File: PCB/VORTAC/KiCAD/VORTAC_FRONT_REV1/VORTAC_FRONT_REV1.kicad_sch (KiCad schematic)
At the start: 5 parts, among them J1 Conn_02x02_Odd_Even, J2 Conn_02x03_Odd_Even, J3 Conn_01x07

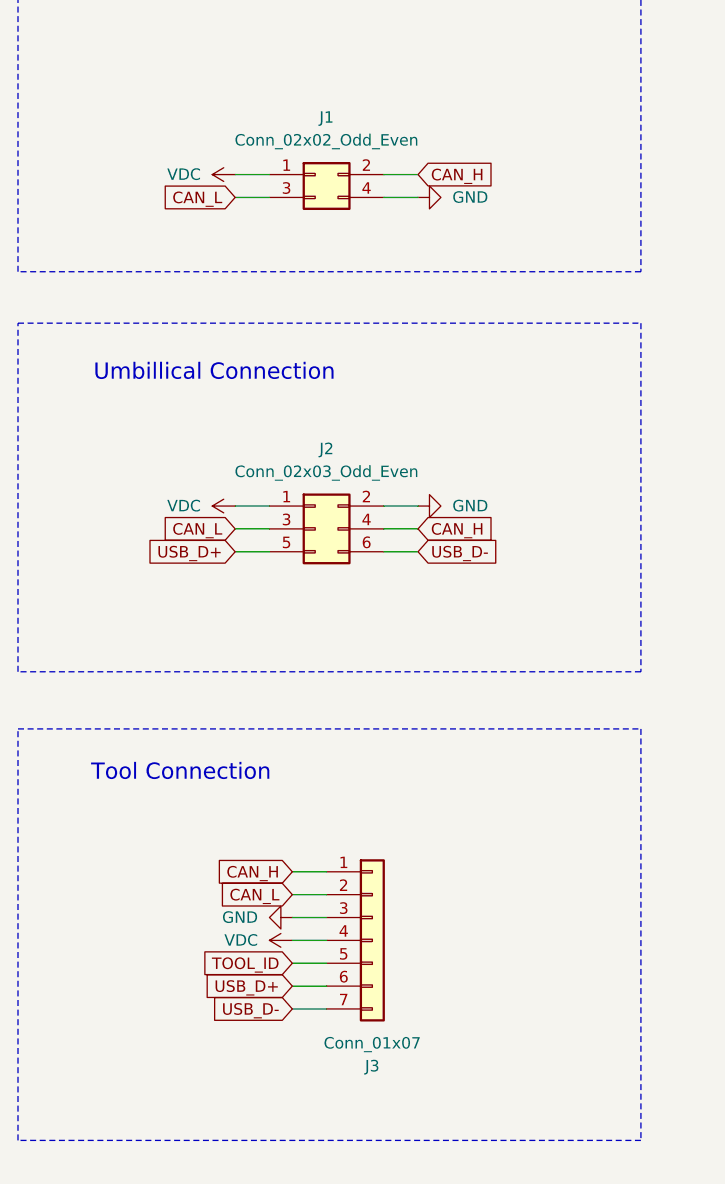
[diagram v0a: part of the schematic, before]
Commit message: No Body knows.... The trouble I've seen
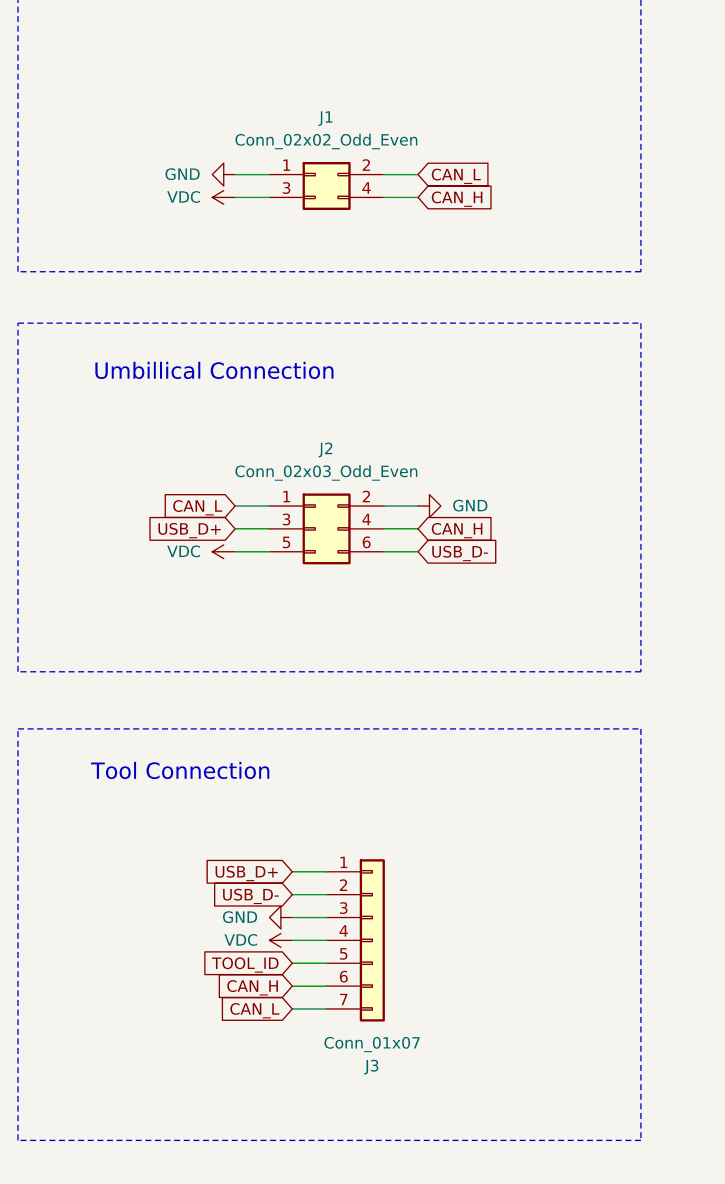
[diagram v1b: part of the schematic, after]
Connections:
- net CAN_H: now also J1.4 (Pin_4), J3.6 (Pin_6); no longer J1.2 (Pin_2), J3.1 (Pin_1)
- net CAN_L: now also J1.2 (Pin_2), J2.1 (Pin_1), J3.7 (Pin_7); no longer J1.3 (Pin_3), J2.3 (Pin_3), J3.2 (Pin_2)
- net GND: now also J1.1 (Pin_1); no longer J1.4 (Pin_4)
- net USB_D+: now also J2.3 (Pin_3), J3.1 (Pin_1); no longer J2.5 (Pin_5), J3.6 (Pin_6)
- net USB_D-: now also J3.2 (Pin_2); no longer J3.7 (Pin_7)
- net VDC: now also J1.3 (Pin_3), J2.5 (Pin_5); no longer J1.1 (Pin_1), J2.1 (Pin_1)

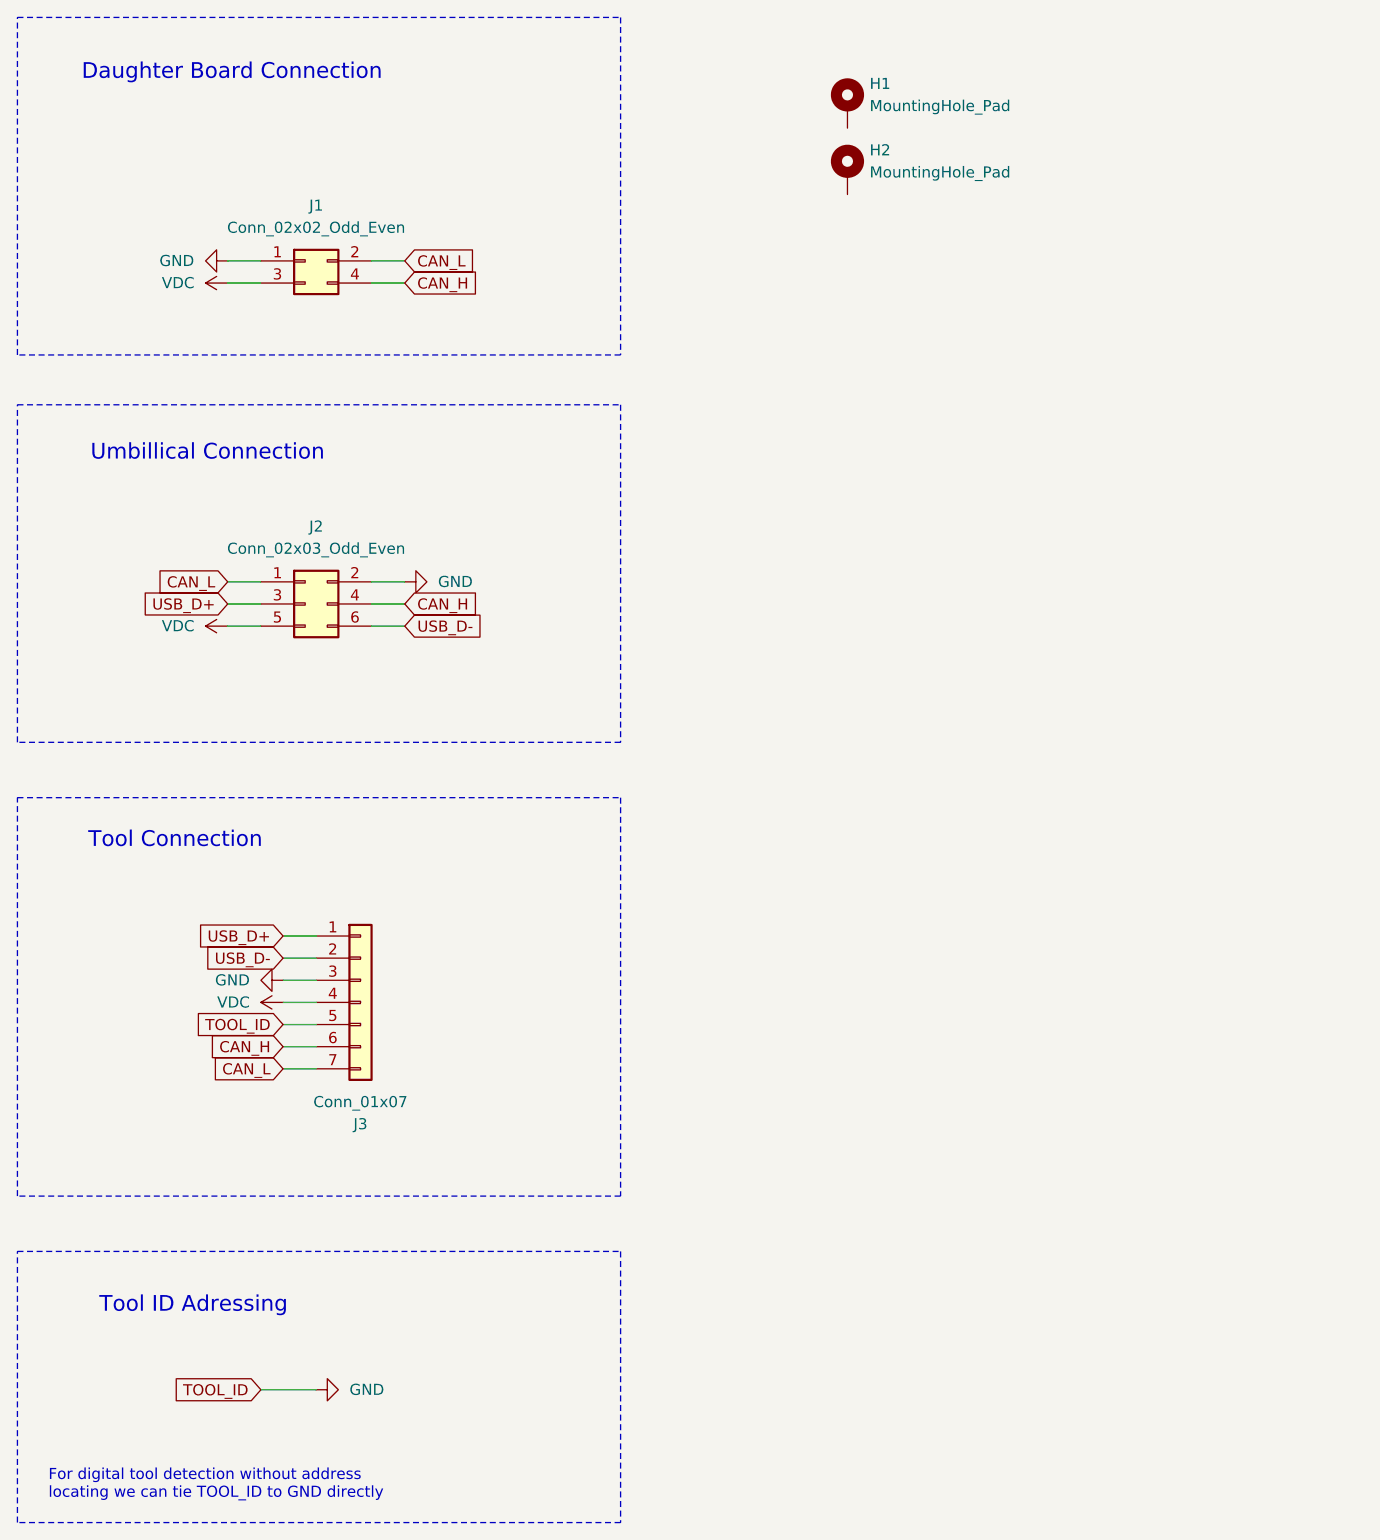
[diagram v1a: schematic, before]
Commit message: FML
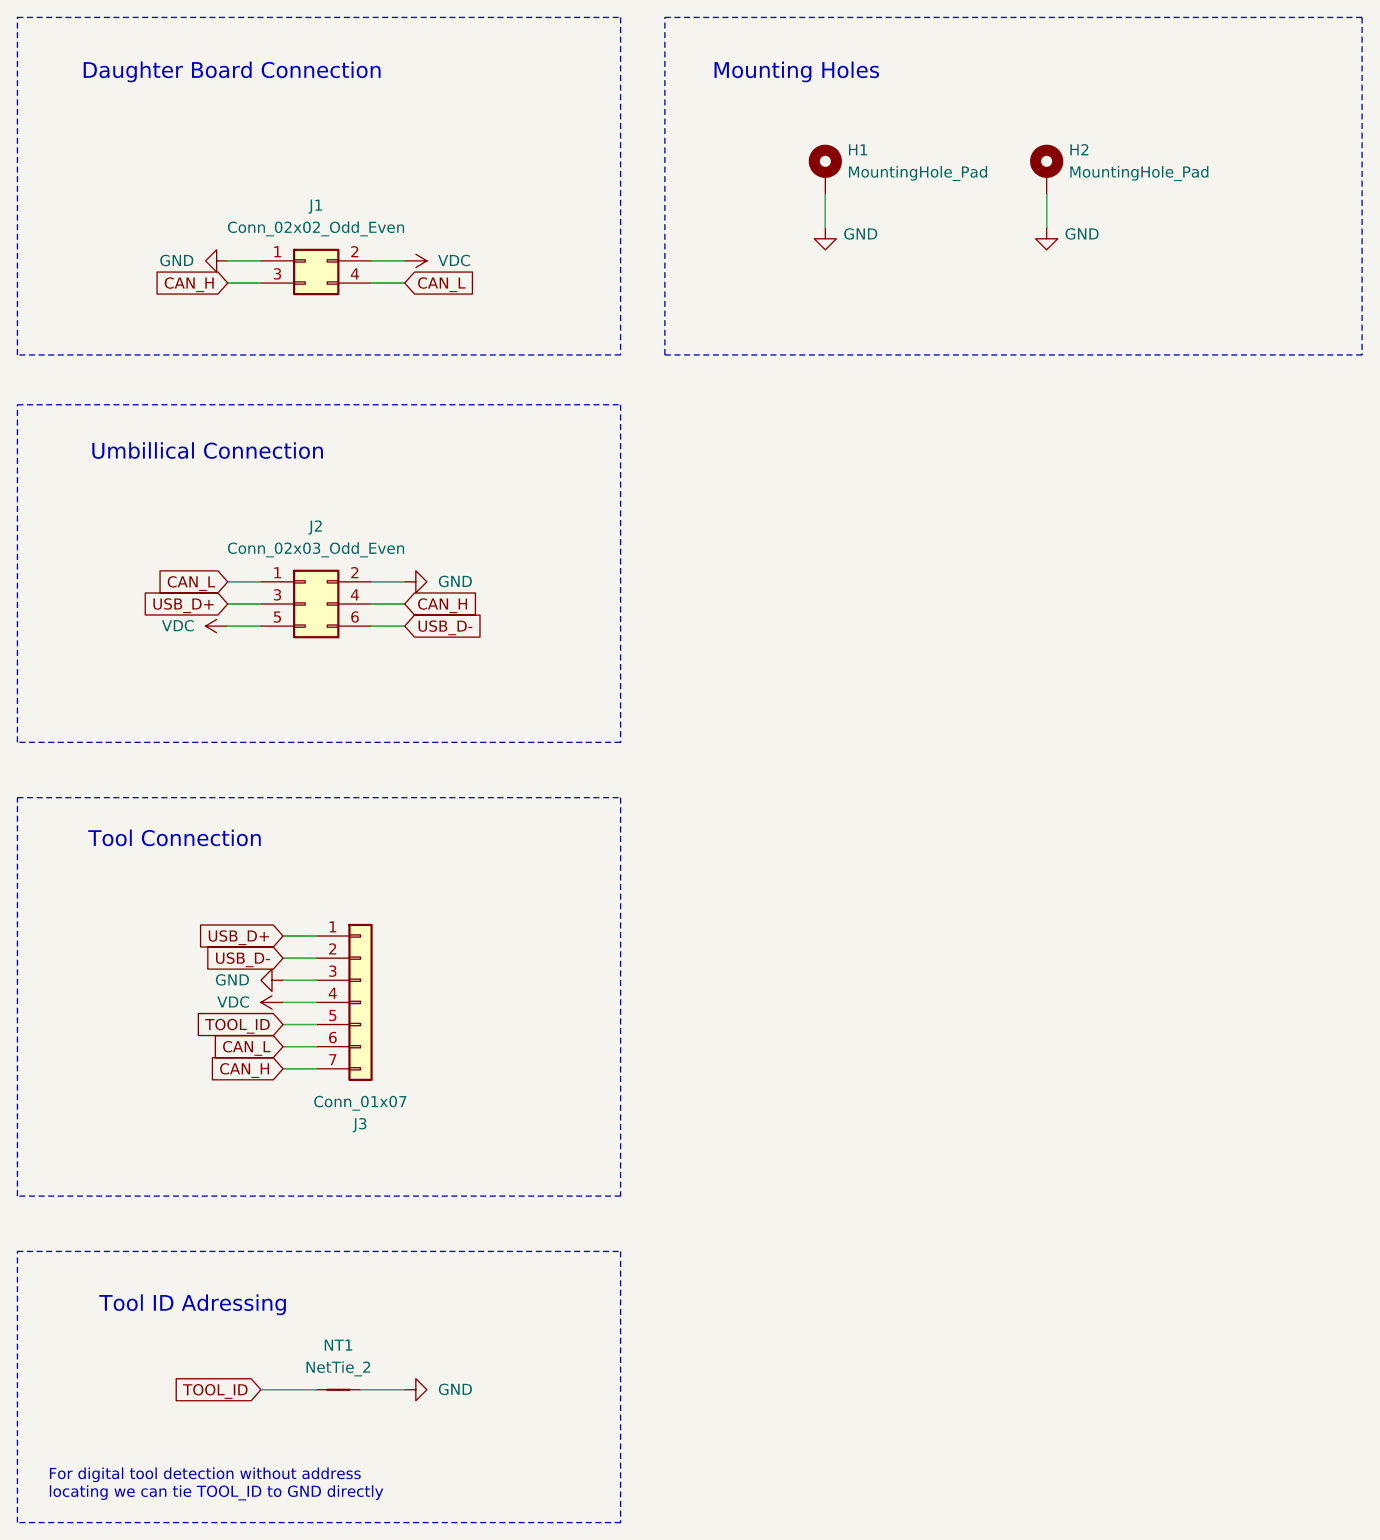
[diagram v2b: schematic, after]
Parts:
- added NT1: NetTie_2, NetTie:NetTie-2_SMD_Pad0.5mm, symbol Device:NetTie_2
- H1, H2: footprint MountingHole:MountingHole_2.2mm_M2_Pad_Via -> Vortac:MountingHole_2.2mm_M2_Pad_Via_NTR
- J1: LCSC (none) -> C2840016
- J2: LCSC (none) -> C234188
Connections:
- net CAN_H: now also J1.3 (Pin_3), J3.7 (Pin_7); no longer J1.4 (Pin_4), J3.6 (Pin_6)
- net CAN_L: now also J1.4 (Pin_4), J3.6 (Pin_6); no longer J1.2 (Pin_2), J3.7 (Pin_7)
- net GND: now also H1.1, H2.1, NT1.2; no longer J3.5 (Pin_5)
- net VDC: now also J1.2 (Pin_2); no longer J1.3 (Pin_3)
- new net TOOL_ID: J3.5 (Pin_5), NT1.1
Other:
- note added: "Mounting Holes"
- moved on the sheet: H1, H2
